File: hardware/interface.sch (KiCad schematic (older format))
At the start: 66 parts, among them J46 Conn_01x03, J47 Conn_01x03, J60 USB_C_Receptacle, J62 Conn_01x02, J66 Conn_01x03, J67 Conn_01x03, J71 Conn_01x02, J72 Conn_01x02, J73 Conn_01x02, J74 Conn_01x02, Q2 AO3401, U5 MAX6675

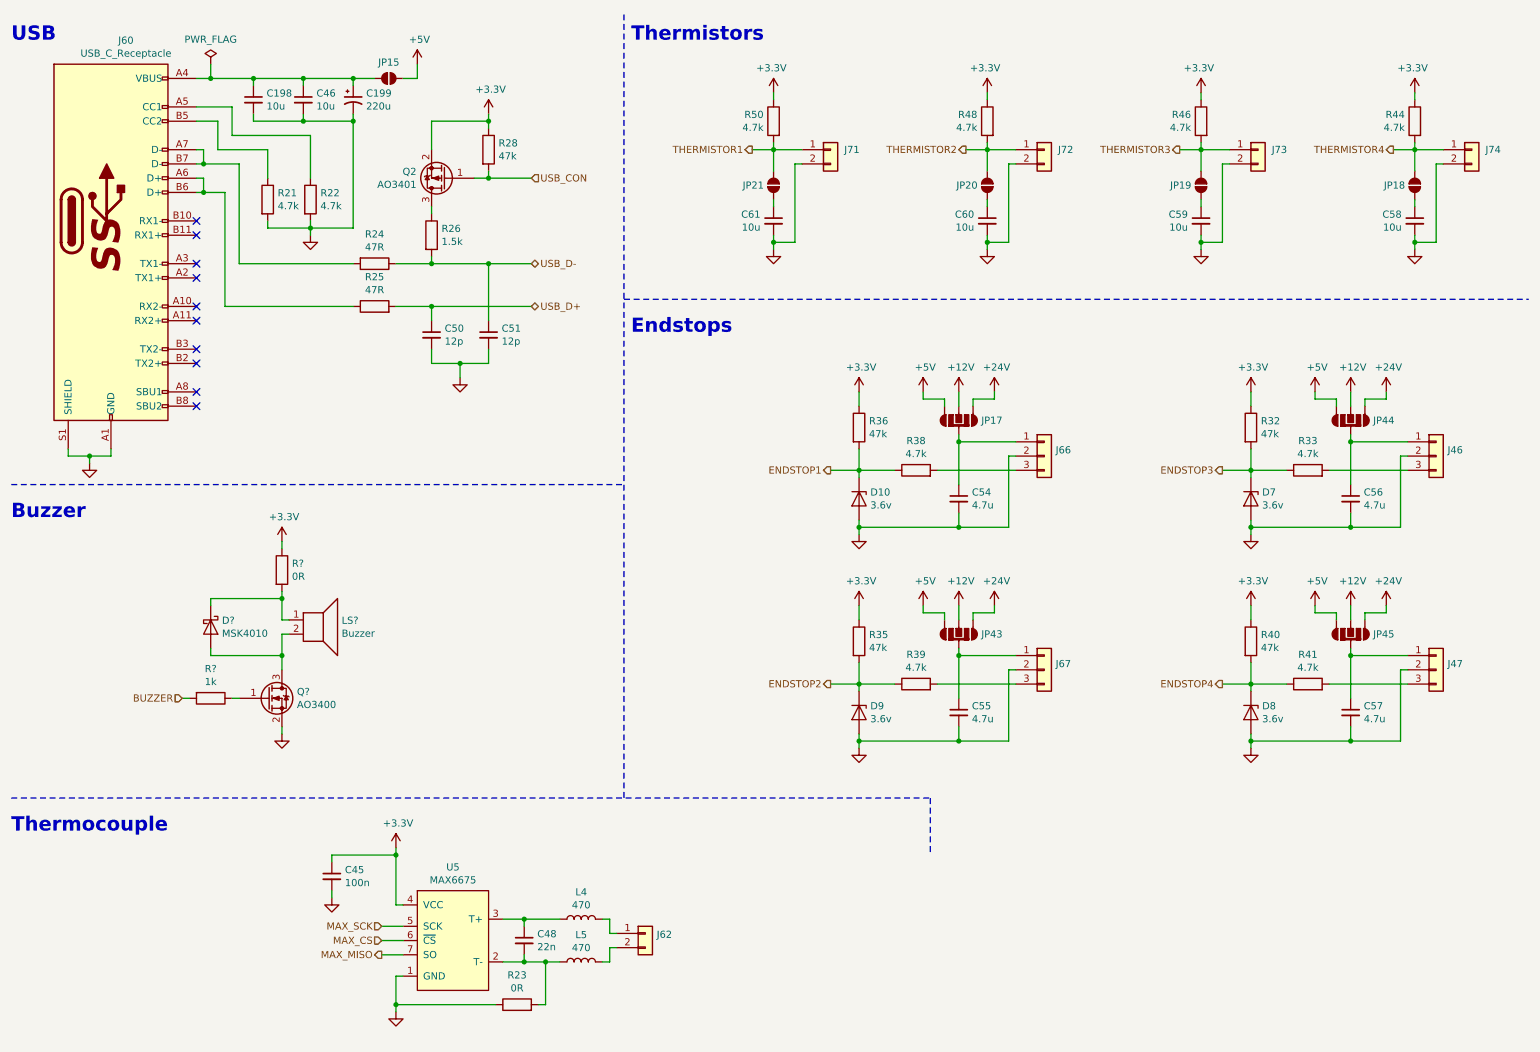
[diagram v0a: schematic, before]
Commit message: layout
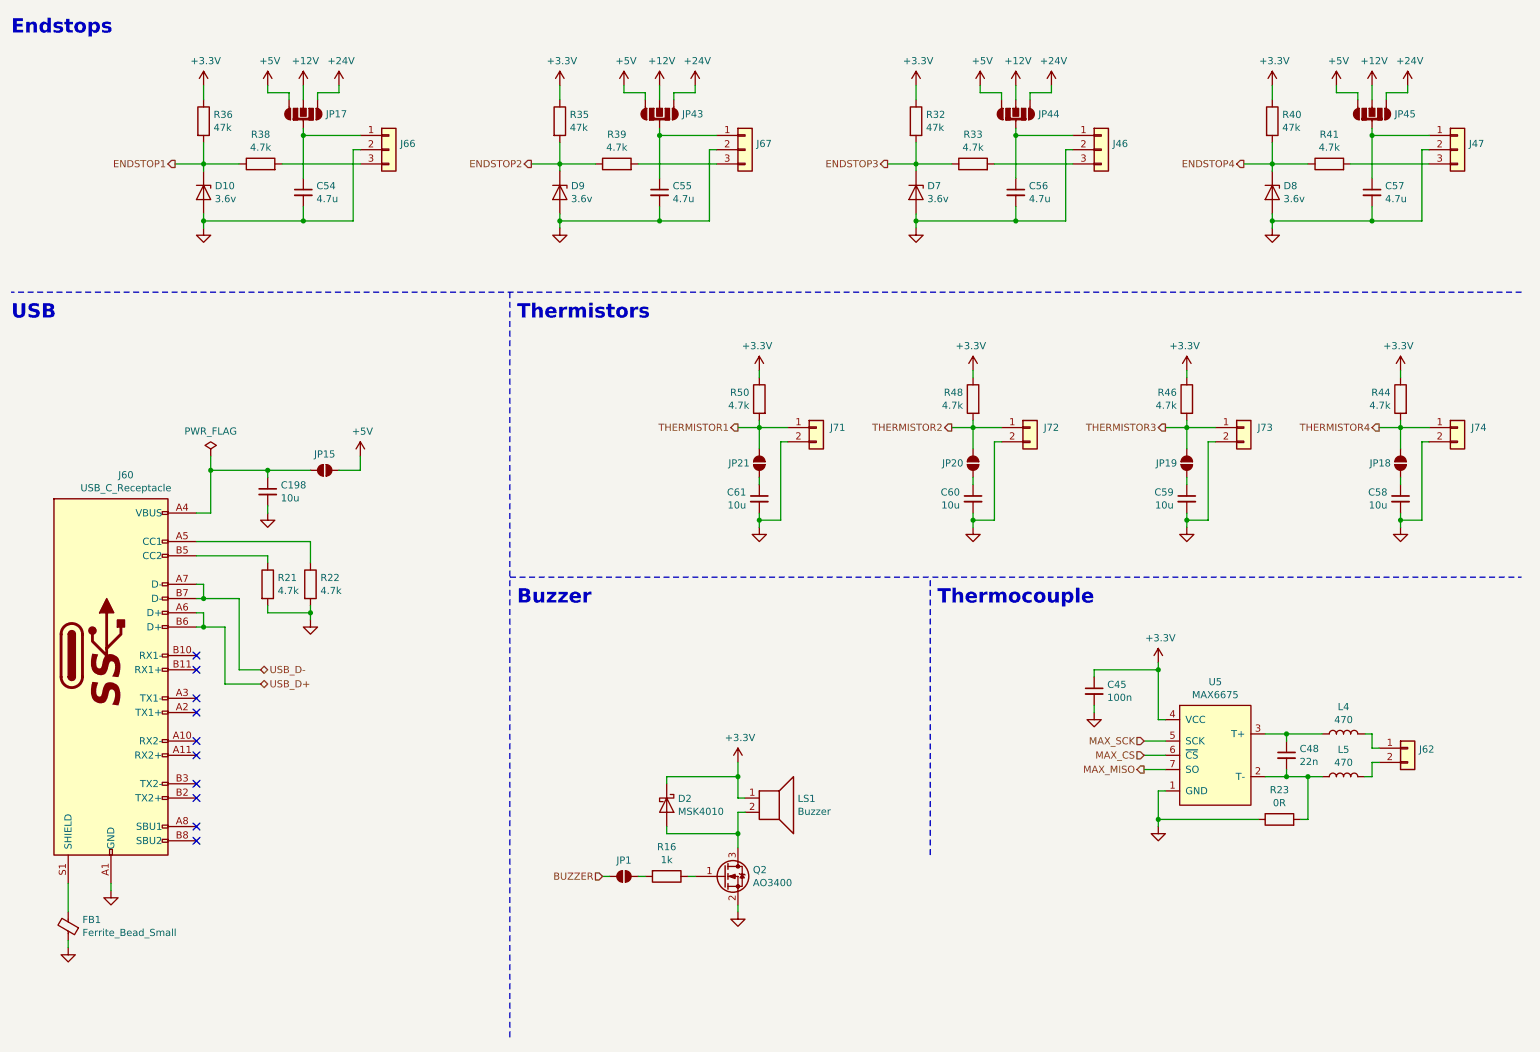
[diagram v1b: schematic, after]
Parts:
- removed C199: 220u, Capacitor_SMD:CP_Elec_6.3x7.7, symbol Device:CP1_Small
- removed C46: 10u, _Generic:0603_CAP, symbol Device:C_Small
- removed C50, C51: 12p, _Generic:0603_CAP, symbol Device:C_Small
- removed Q2: AO3401, _Generic:SOT-23, symbol Device:Q_PMOS_GSD
- removed R24, R25: 47R, _Generic:0603_RES, symbol Device:R
- removed R26: 1.5k, _Generic:0603_RES, symbol Device:R
- removed R28: 47k, _Generic:0603_RES, symbol Device:R
- removed R?: 0R, _Generic:0603_RES, symbol Device:R
- added FB1: Ferrite_Bead_Small, _Generic:0805_IND, symbol Device:Ferrite_Bead_Small
- added JP1: SolderJumper_2_Open, _Generic:Solder Jumper 2P, symbol #PCB_Only:SolderJumper_2_Open
- gave numbers to parts that had none: 4
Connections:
- net +3V3: now also D2.1 (K), LS1.1
- net BUZZER: now also JP1.1 (A); no longer R16.2
- net GND: now also FB1.1; no longer J60.S1 (SHIELD)
- net USB_D+: now also J60.A6 (D+), J60.B6 (D+)
- net USB_D-: now also J60.A7 (D-), J60.B7 (D-)
- new net: FB1.2, J60.S1 (SHIELD)
- new net: JP1.2 (B), R16.2
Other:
- moved on the sheet: C198, C45, C48, C54, C55, C56, C57, C58, C59, C60, C61, D10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

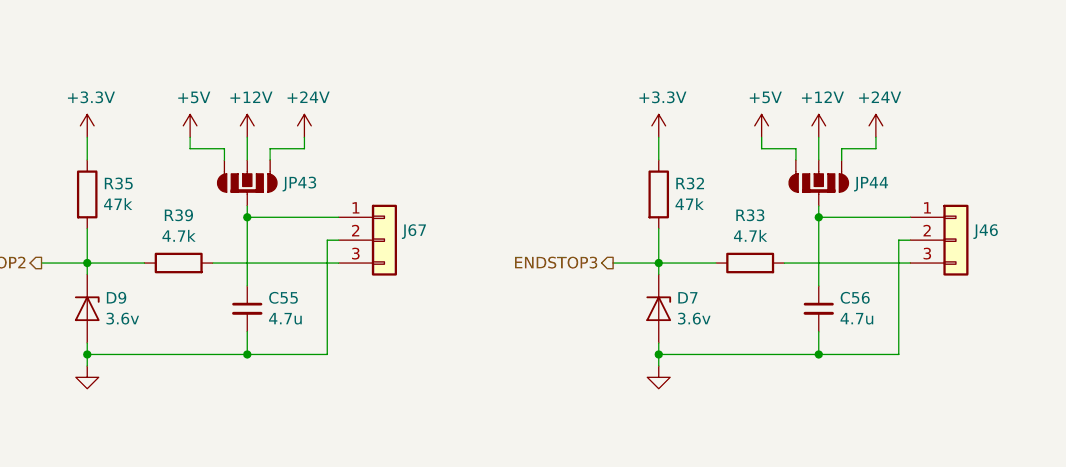
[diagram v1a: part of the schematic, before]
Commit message: layout
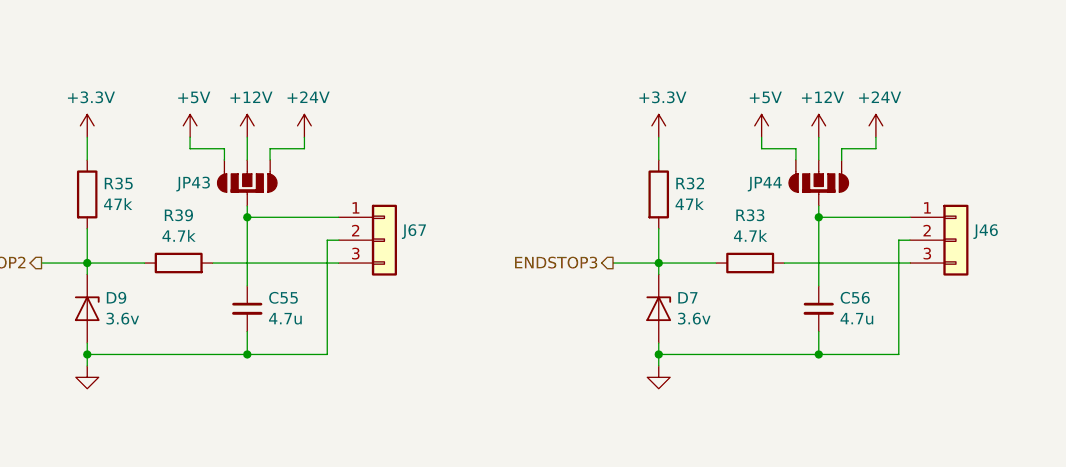
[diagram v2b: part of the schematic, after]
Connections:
- net +24V: now also JP43.2 (O1), JP44.2 (O1); no longer JP43.4 (O4), JP44.4 (O4)
- net +5V: now also JP43.4 (O4), JP44.4 (O4); no longer JP43.2 (O1), JP44.2 (O1)
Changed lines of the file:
@@
 F 3 "~" H 5100 1250 50  0001 C CNN
 	1    5100 1250
-	1    0    0    -1
+	-1   0    0    -1
 $EndComp
 $Comp
@@
 F 3 "~" H 7600 1250 50  0001 C CNN
 	1    7600 1250
-	1    0    0    -1
+	-1   0    0    -1
 $EndComp
 $Comp

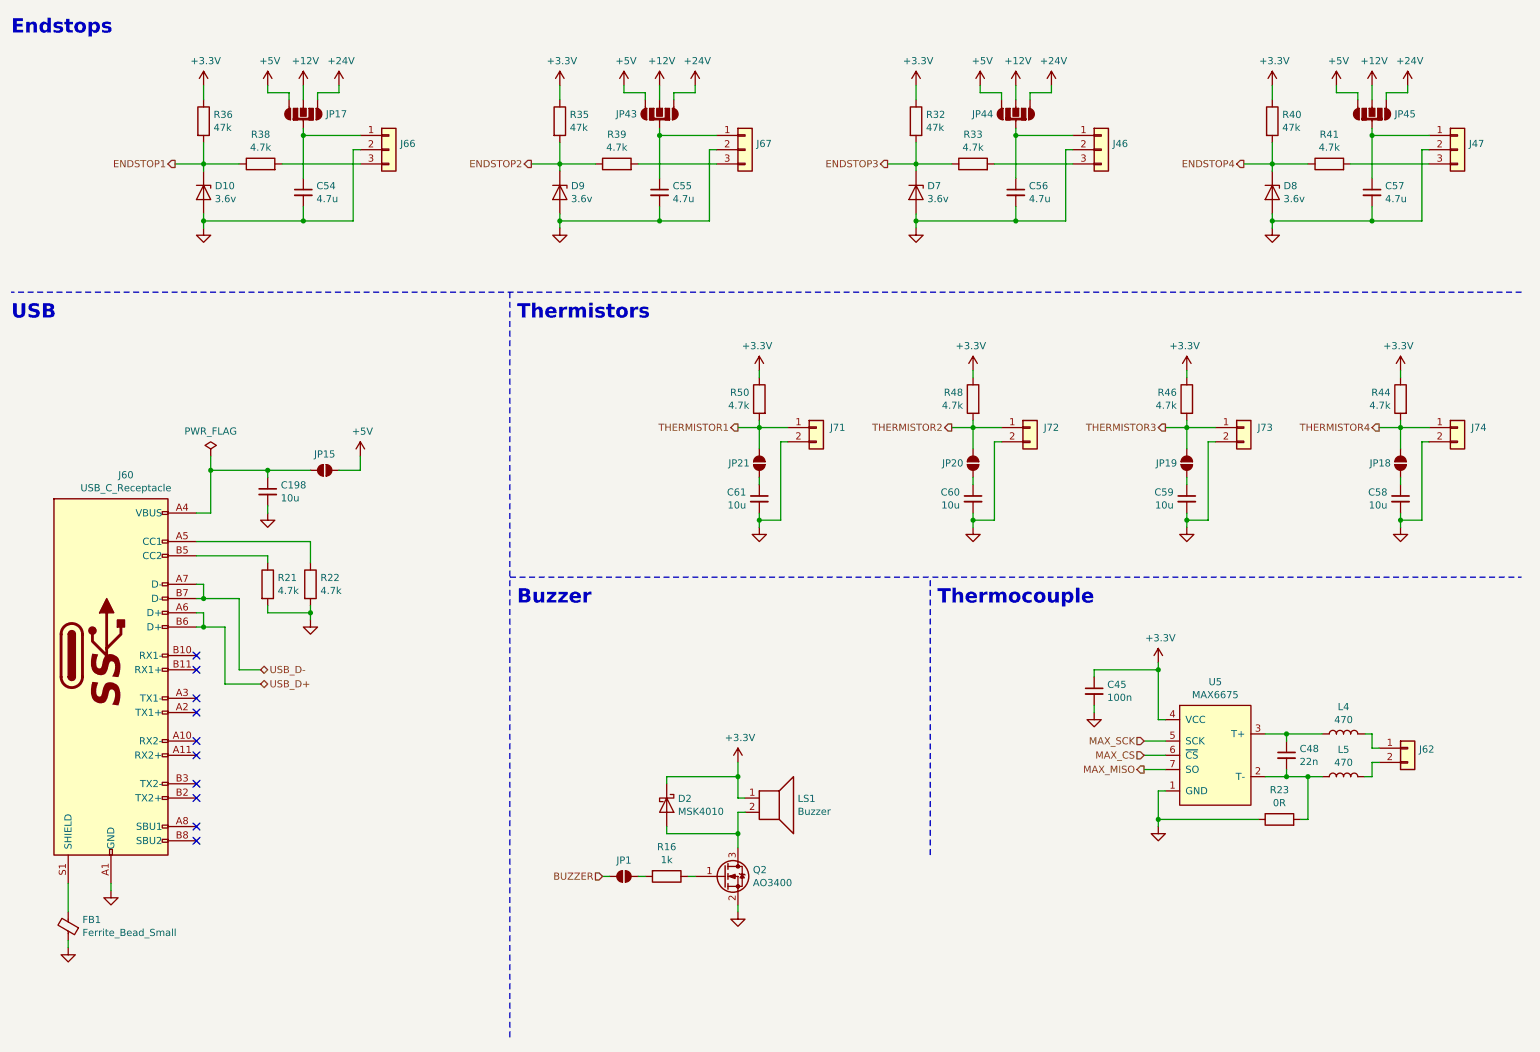
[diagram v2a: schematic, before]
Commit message: combine
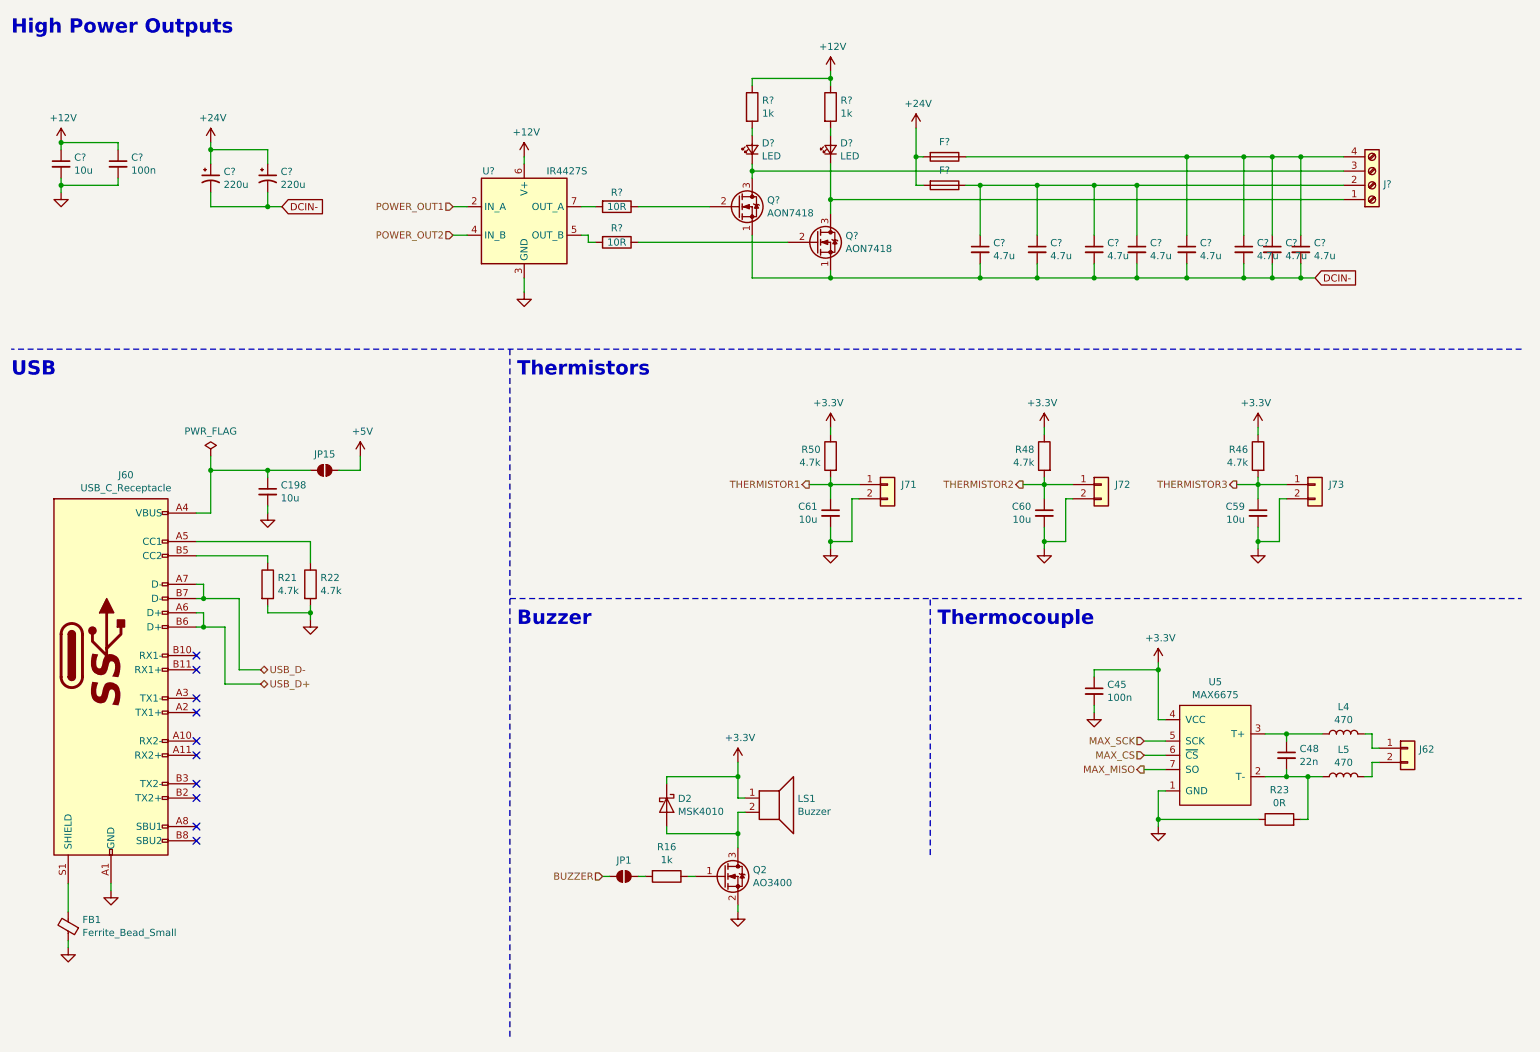
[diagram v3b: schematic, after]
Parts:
- removed C54, C55, C56, C57: 4.7u, _Generic:0805_CAP, symbol Device:C_Small
- removed C58: 10u, _Generic:0603_CAP, symbol Device:C_Small
- removed D10, D7, D8, D9: 3.6v, _Generic:SOD-523_DIODE, symbol Device:D_Zener
- removed J46, J47, J66, J67: Conn_01x03, _Generic:JST_XH_3P, symbol Connector_Generic:Conn_01x03
- removed J74: Conn_01x02, _Generic:JST_XH_2P, symbol Connector_Generic:Conn_01x02
- removed JP17, JP43, JP44, JP45: SolderJumper_4_Open, _Generic:SolderJumper_JST, symbol #PCB_Only:SolderJumper_4_Open
- removed JP18, JP19, JP20, JP21: SolderJumper_2_Open, _Generic:Solder Jumper 2P, symbol #PCB_Only:SolderJumper_2_Open
- removed R32, R35, R36, R40: 47k, _Generic:0603_RES, symbol Device:R
- removed R33, R38, R39, R41, R44: 4.7k, _Generic:0603_RES, symbol Device:R
- added C?: 100n, _Generic:0603_CAP, symbol Device:C_Small
- added C?: 10u, _Generic:0603_CAP, symbol Device:C_Small
- added C? (x2): 220u, Capacitor_SMD:CP_Elec_6.3x7.7, symbol Device:CP1_Small
- added C? (x8): 4.7u, _Generic:1210_CAP, symbol Device:C_Small
- added D? (x2): LED, _Generic:0603_LED, symbol Device:LED_Small
- added F? (x2): Fuse, _Generic:1206_RES, symbol Device:Fuse
- added J?: Screw_Terminal_01x04, _Generic:KF635-4P, symbol Connector:Screw_Terminal_01x04
- added Q? (x2): AON7418, _Generic:DFN3x3A_8L_EP1_P, symbol Device:Q_NMOS_SGD
- added R? (x2): 10R, _Generic:0603_RES, symbol Device:R
- added R? (x2): 1k, _Generic:0603_RES, symbol Device:R
- added U?: IR4427S, _Generic:SO-8, symbol Driver_FET:MIC4427
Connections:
- net +12V: now also C?.1, C?.1, R?.1, R?.1, U?.6 (V+)
- net +24V: now also C?.1, C?.1, F?.2, F?.2
- net GND: now also C?.2, C?.2, U?.3 (GND)
- net THERMISTOR1: now also C61.1
- net THERMISTOR2: now also C60.1
- net THERMISTOR3: now also C59.1
- new net: D?.1 (K), J?.1 (Pin_1), Q?.3 (D)
- new net: C?.1, C?.1, C?.1, C?.1, F?.1, J?.2 (Pin_2)
- new net: D?.1 (K), J?.3 (Pin_3), Q?.3 (D)
- new net: C?.1, C?.1, C?.1, C?.1, F?.1, J?.4 (Pin_4)
- new net: Q?.2 (G), R?.1 (x2)
- new net: R?.2, U?.5 (OUT_B)
- new net: R?.2, U?.7 (OUT_A)
- new net: D?.2 (A), R?.2 (x2)
- new net DCIN-: C?.2, C?.2, C?.2, C?.2, C?.2, C?.2, C?.2, C?.2, C?.2, C?.2, Q?.1 (S), Q?.1 (S)
- new net POWER_OUT1: U?.2 (IN_A)
- new net POWER_OUT2: U?.4 (IN_B)
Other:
- note added: "High Power Outputs"
- note removed: "Endstops"
- moved on the sheet: C59, C60, C61, J71, J72, J73, R46, R48, R50
